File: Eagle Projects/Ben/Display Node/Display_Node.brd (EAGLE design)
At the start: 93 x 90 mm, 90 parts, among them Q1 16MHz, Q3 16MHz, Q4 16MHz, Q5 16MHz, Q6 2N7002, Q7 2N7002, U1 ATMEGA328P_TQFP, U2 MCP2551, X1 5566-6, X2 5566-6

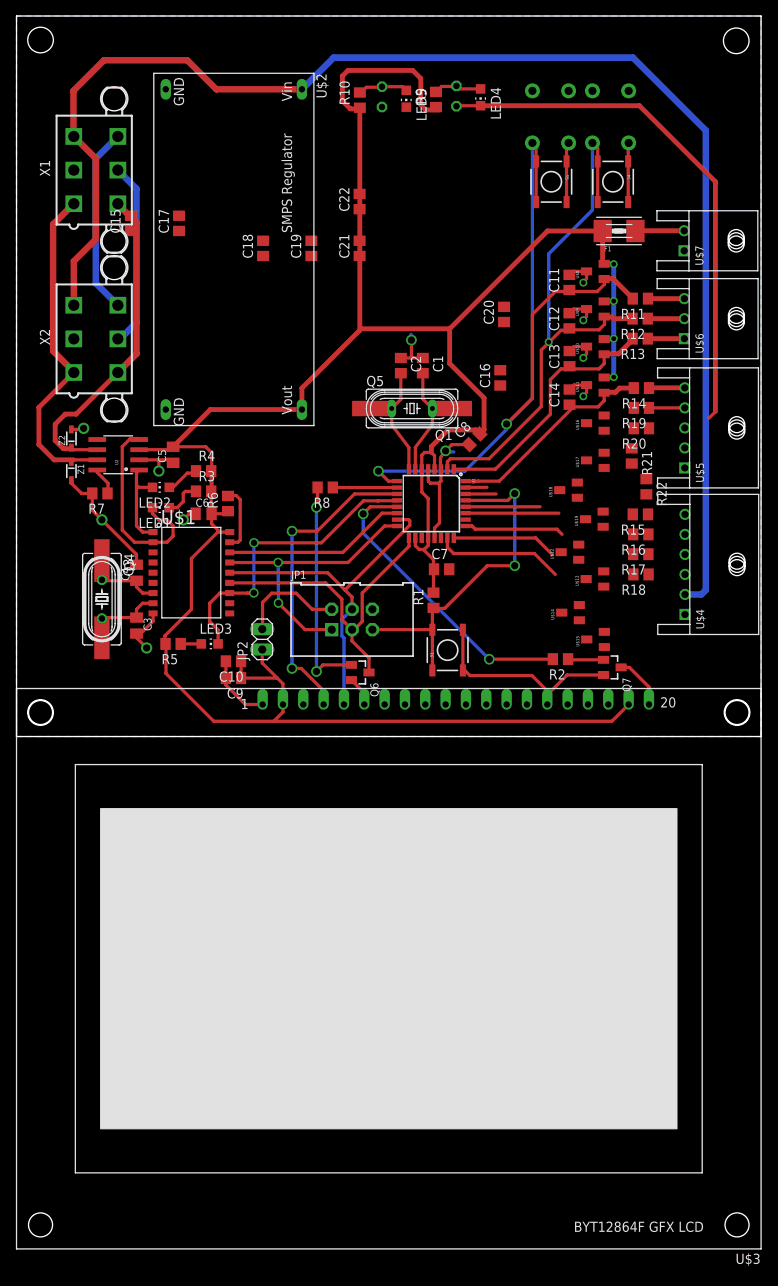
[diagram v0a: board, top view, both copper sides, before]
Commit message: Display Node Done?
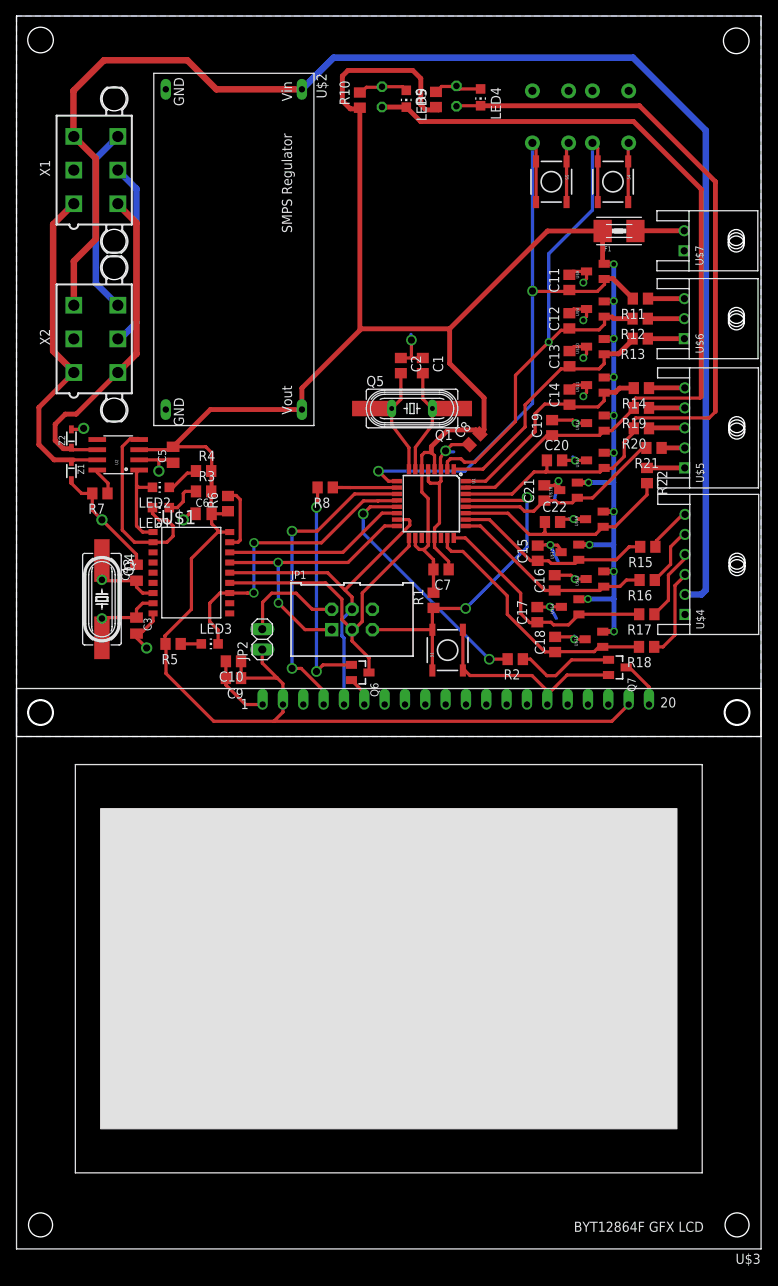
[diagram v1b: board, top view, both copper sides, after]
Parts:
- moved C17 66.3 mm to (65.0, 15.2)
- moved C15 65.4 mm to (65.1, 22.9)
- moved C18 61.5 mm to (67.3, 11.5)
- moved C22 46.7 mm to (67.0, 26.8), turned to 0 degrees
- moved C21 38.3 mm to (65.9, 30.4)
- moved C19 37.5 mm to (66.9, 38.6)
- moved C16 26.5 mm to (67.2, 19.2)
- moved C20 19.3 mm to (67.2, 34.5), turned to 0 degrees
- moved R18 9.08 mm to (78.7, 11.2)
- moved R17 7.54 mm to (78.7, 15.3)
- moved R16 5.76 mm to (78.8, 19.6)
- moved R2 5.65 mm to (62.3, 9.67)
- moved R15 4.15 mm to (78.8, 23.7)
- moved R21 2.95 mm to (79.6, 36.0), turned to 180 degrees
- moved R22 1.40 mm to (78.8, 32.6)
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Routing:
- net LED2: track 2.67 -> 104.8 mm
- net +5V: track 313.7 -> 366.2 mm, vias 4 -> 12
- net GND: track 121.0 -> 165.6 mm, vias 11 -> 19
- net LED1: track 69.9 -> 104.0 mm
- net CRUISE4: track 0.00 -> 24.9 mm
- net A0: track 11.6 -> 28.9 mm
- net A1: track 9.29 -> 26.3 mm
- net CRUISE2: track 13.1 -> 29.7 mm
- net BTN4: track 96.9 -> 80.7 mm
- net CRUISE1: track 16.0 -> 32.1 mm
- net CRUISE3: track 12.5 -> 25.9 mm
- net N$22: track 0.00 -> 11.3 mm
- net N$23: track 0.00 -> 9.06 mm
- net N$5: track 4.53 -> 12.4 mm
- net N$24: track 0.00 -> 7.41 mm
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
